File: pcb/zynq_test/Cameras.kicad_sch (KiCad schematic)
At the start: 46 parts, among them J1201 1-1734248-5, J1202 1-1734248-5, J1203 Conn_02x04_Odd_Even, J1204 1-1734248-5

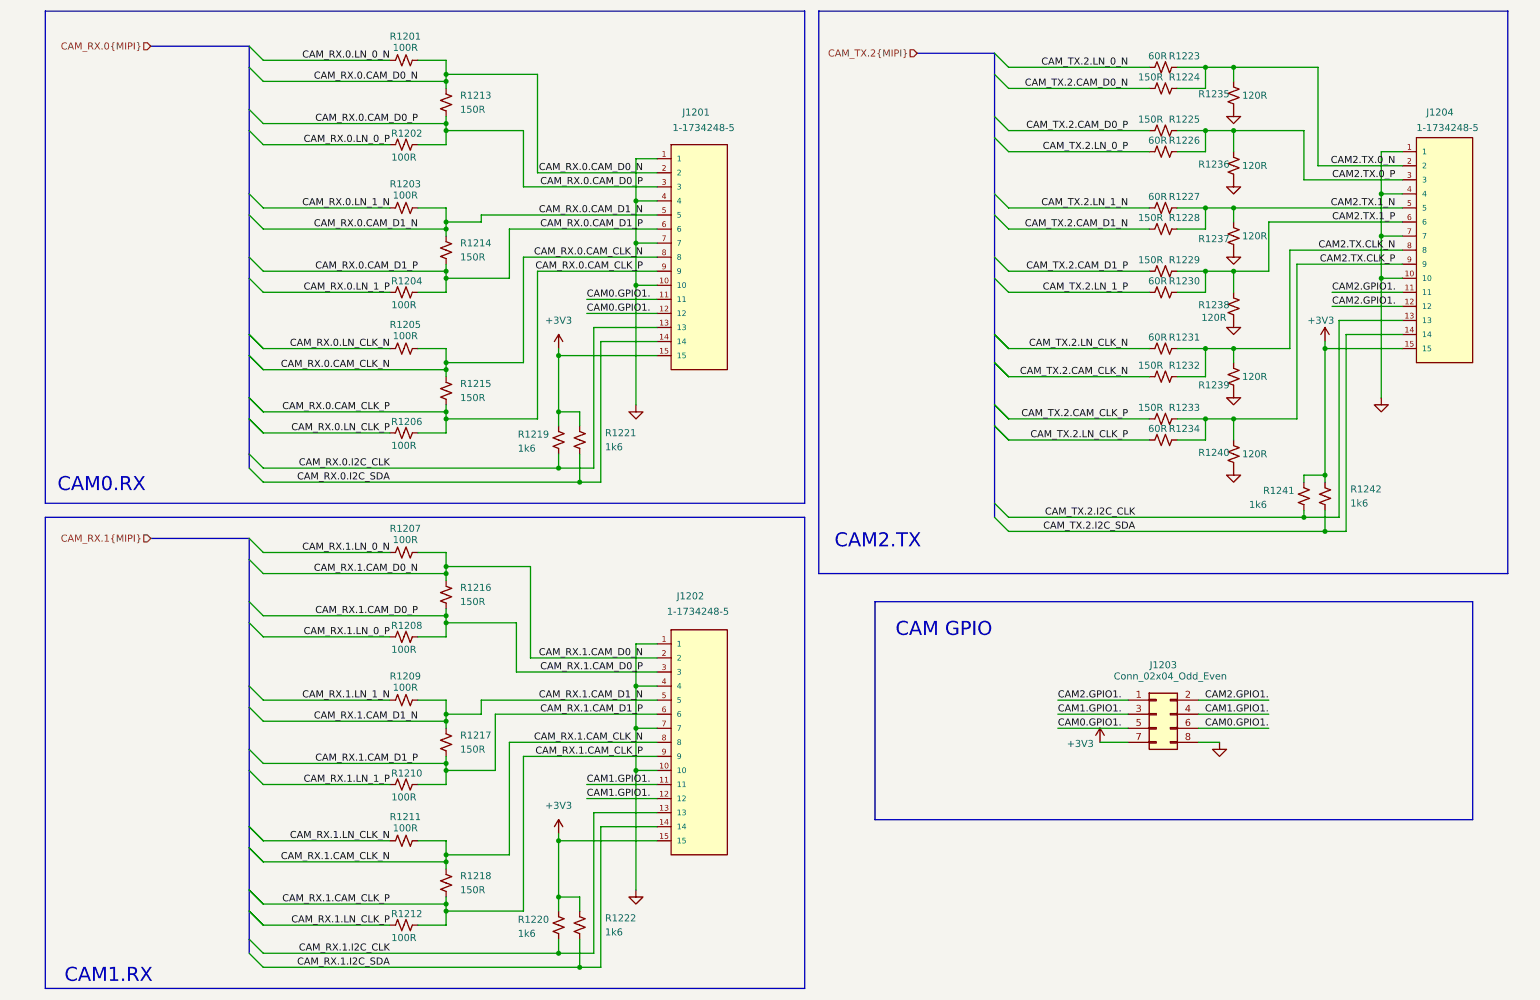
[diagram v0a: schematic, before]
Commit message: Almost done with BOM
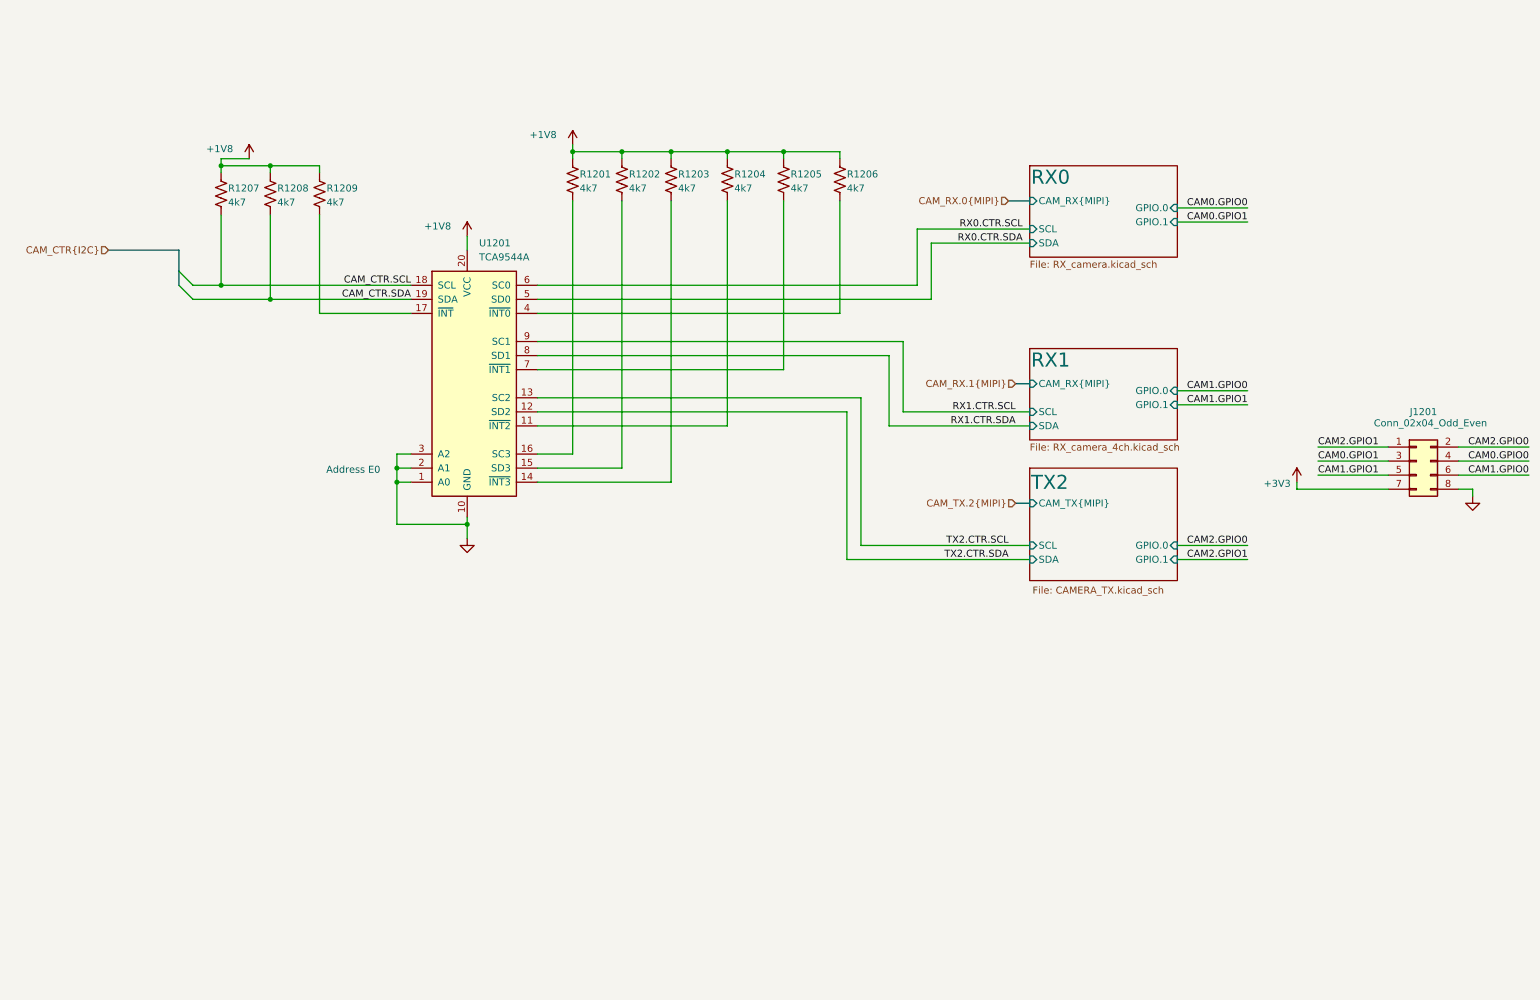
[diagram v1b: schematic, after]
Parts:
- removed J1201, J1202, J1204: 1-1734248-5, symbol camera:1-1734248-5
- removed R1201, R1202, R1203, R1204, R1205, R1206, R1207, R1208, R1209, R1210, R1211, R1212: 100R, Resistor_SMD:R_0402_1005Metric, symbol Device:R_Small_US
- removed R1213, R1214, R1215, R1216, R1217, R1218, R1224, R1225, R1228, R1229, R1232, R1233: 150R, Resistor_SMD:R_0402_1005Metric, symbol Device:R_Small_US
- removed R1219, R1220, R1221, R1222, R1241, R1242: 1k6, Resistor_SMD:R_0402_1005Metric, symbol Device:R_Small_US
- removed R1223, R1226, R1227, R1230, R1231, R1234: 60R, Resistor_SMD:R_0402_1005Metric, symbol Device:R_Small_US
- removed R1235, R1236, R1237, R1238, R1239, R1240: 120R, Resistor_SMD:R_0402_1005Metric, symbol Device:R_Small_US
- added R1201, R1202, R1203, R1204, R1205, R1206, R1207, R1208, R1209: 4k7, Resistor_SMD:R_0402_1005Metric, symbol Device:R_US
- added U1201: TCA9544A, Package_SO:TSSOP-20_4.4x6.5mm_P0.65mm, symbol Interface_Expansion:TCA9544A
- J1201: renamed from J1203; footprint (none) -> Connector_PinSocket_1.27mm:PinSocket_2x04_P1.27mm_Vertical_SMD
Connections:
- net GND: now also U1201.1 (A0), U1201.10 (GND), U1201.2 (A1), U1201.3 (A2)
- net CAM0.GPIO1. renamed CAM1.GPIO0
- net CAM1.GPIO0: no longer J1201.5 (Pin_5)
- net CAM1.GPIO1. renamed CAM0.GPIO0
- net CAM0.GPIO0: no longer J1201.3 (Pin_3)
- net CAM2.GPIO1. renamed CAM2.GPIO0
- net CAM2.GPIO0: no longer J1201.1 (Pin_1)
- new net: R1203.2, U1201.14 (~{INT3})
- new net: R1204.2, U1201.11 (~{INT2})
- new net: R1202.2, U1201.15 (SD3)
- new net: R1201.2, U1201.16 (SC3)
- new net: R1209.2, U1201.17 (~{INT})
- new net: R1206.2, U1201.4 (~{INT0})
- new net: R1205.2, U1201.7 (~{INT1})
- new net +1V8: R1201.1, R1202.1, R1203.1, R1204.1, R1205.1, R1206.1, R1207.1, R1208.1, R1209.1, U1201.20 (VCC)
- new net CAM0.GPIO1: J1201.3 (Pin_3)
- new net CAM1.GPIO1: J1201.5 (Pin_5)
- new net CAM2.GPIO1: J1201.1 (Pin_1)
- new net CAM_CTR.SCL: R1207.2, U1201.18 (SCL)
- new net CAM_CTR.SDA: R1208.2, U1201.19 (SDA)
- new net RX0.CTR.SCL: U1201.6 (SC0)
- new net RX0.CTR.SDA: U1201.5 (SD0)
- new net RX1.CTR.SCL: U1201.9 (SC1)
- new net RX1.CTR.SDA: U1201.8 (SD1)
- new net TX2.CTR.SCL: U1201.13 (SC2)
- new net TX2.CTR.SDA: U1201.12 (SD2)
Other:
- added sheet RX0 (RX_camera.kicad_sch)
- added sheet RX1 (RX_camera_4ch.kicad_sch)
- added sheet TX2 (CAMERA_TX.kicad_sch)
- note added: "Address E0"
- note removed: "CAM GPIO"
- note removed: "CAM0.RX"
- note removed: "CAM1.RX"
- note removed: "CAM2.TX"
- moved on the sheet: J1201

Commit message: Version sent to JLCPCB
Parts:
- J1201: now left out of the parts list
- R1201, R1202, R1203, R1204, R1205, R1206, R1207, R1208, R1209: JLCPCB Part# (none) -> C327817; PART_NUMBER (none) -> MR04X4701FTL
- U1201: JLCPCB Part# (none) -> C2674619; PART_NUMBER (none) -> TCA9544APWR
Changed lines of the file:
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@@
+			)
+		)
+		(property "PART_NUMBER" "MR04X4701FTL"
+			(at 130.81 49.53 0)
+			(effects
+				(font
+					(size 1.27 1.27)
+				)
+				(hide yes)
+			)
+		)
+		(property "JLCPCB Part#" "C327817"
+			(at 130.81 49.53 0)
+			(effects
+				(font
+					(size 1.27 1.27)
+				)
+				(hide yes)
 			)
 		)
@@
 			)
 		)
+		(property "PART_NUMBER" "TCA9544APWR"
+			(at 93.98 86.36 0)
+			(effects
+				(font
+					(size 1.27 1.27)
+				)
+				(hide yes)
+			)
+		)
+		(property "JLCPCB Part#" "C2674619"
+			(at 93.98 86.36 0)
+			(effects
+				(font
+					(size 1.27 1.27)
+				)
+				(hide yes)
+			)
+		)
 		(pin "17"
 		)
@@
 			)
 		)
+		(property "PART_NUMBER" "MR04X4701FTL"
+			(at 151.13 49.53 0)
+			(effects
+				(font
+					(size 1.27 1.27)
+				)
+				(hide yes)
+			)
+		)
+		(property "JLCPCB Part#" "C327817"
+			(at 151.13 49.53 0)
+			(effects
+				(font
+					(size 1.27 1.27)
+				)
+				(hide yes)
+			)
+		)
 		(pin "2"
 		)
@@
 		)
 		(property "Description" "Resistor, US symbol"
+			(at 49.53 52.07 0)
+			(effects
+				(font
+					(size 1.27 1.27)
+				)
+				(hide yes)
+			)
+		)
+		(property "PART_NUMBER" "MR04X4701FTL"
+			(at 49.53 52.07 0)
+			(effects
+				(font
+					(size 1.27 1.27)
+				)
+				(hide yes)
+			)
+		)
+		(property "JLCPCB Part#" "C327817"
 			(at 49.53 52.07 0)
 			(effects
@@
 			)
 		)
+		(property "PART_NUMBER" "MR04X4701FTL"
+			(at 121.92 49.53 0)
+			(effects
+				(font
+					(size 1.27 1.27)
+				)
+				(hide yes)
+			)
+		)
+		(property "JLCPCB Part#" "C327817"
+			(at 121.92 49.53 0)
+			(effects
+				(font
+					(size 1.27 1.27)
+				)
+				(hide yes)
+			)
+		)
 		(pin "2"
 		)
@@
 			)
 		)
+		(property "PART_NUMBER" "MR04X4701FTL"
+			(at 113.03 49.53 0)
+			(effects
+				(font
+					(size 1.27 1.27)
+				)
+				(hide yes)
+			)
+		)
+		(property "JLCPCB Part#" "C327817"
+			(at 113.03 49.53 0)
+			(effects
+				(font
+					(size 1.27 1.27)
+				)
+				(hide yes)
+			)
+		)
 		(pin "2"
 		)
@@
 		(unit 1)
 		(exclude_from_sim no)
-		(in_bom yes)
+		(in_bom no)
 		(on_board yes)
 		(dnp no)
@@
 			)
 		)
+		(property "PART_NUMBER" ""
+			(at 265.43 100.33 0)
+			(effects
+				(font
+					(size 1.27 1.27)
+				)
+				(hide yes)
+			)
+		)
+		(property "JLCPCB Part#" ""
+			(at 265.43 100.33 0)
+			(effects
+				(font
+					(size 1.27 1.27)
+				)
+				(hide yes)
+			)
+		)
 		(pin "4"
 		)
@@
 			)
 		)
+		(property "PART_NUMBER" "MR04X4701FTL"
+			(at 140.97 49.53 0)
+			(effects
+				(font
+					(size 1.27 1.27)
+				)
+				(hide yes)
+			)
+		)
+		(property "JLCPCB Part#" "C327817"
+			(at 140.97 49.53 0)
+			(effects
+				(font
+					(size 1.27 1.27)
+				)
+				(hide yes)
+			)
+		)
 		(pin "2"
 		)
@@
 			)
 		)
+		(property "PART_NUMBER" "MR04X4701FTL"
+			(at 58.42 52.07 0)
+			(effects
+				(font
+					(size 1.27 1.27)
+				)
+				(hide yes)
+			)
+		)
+		(property "JLCPCB Part#" "C327817"
+			(at 58.42 52.07 0)
+			(effects
+				(font
+					(size 1.27 1.27)
+				)
+				(hide yes)
+			)
+		)
 		(pin "2"
 		)
@@
 			)
 		)
+		(property "PART_NUMBER" "MR04X4701FTL"
+			(at 67.31 52.07 0)
+			(effects
+				(font
+					(size 1.27 1.27)
+				)
+				(hide yes)
+			)
+		)
+		(property "JLCPCB Part#" "C327817"
+			(at 67.31 52.07 0)
+			(effects
+				(font
+					(size 1.27 1.27)
+				)
+				(hide yes)
+			)
+		)
 		(pin "2"
 		)
@@
 			(at 161.29 49.53 0)
 			(effects
+				(font
+					(size 1.27 1.27)
+				)
+				(hide yes)
+			)
+		)
+		(property "PART_NUMBER" "MR04X4701FTL"
+			(at 161.29 49.53 0)
+			(effects
+				(font
+					(size 1.27 1.27)
+				)
+				(hide yes)
+			)
+		)
+		(property "JLCPCB Part#" "C327817"
+			(at 161.29 49.53 0)
+			(effects
